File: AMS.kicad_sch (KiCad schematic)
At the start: 1 part

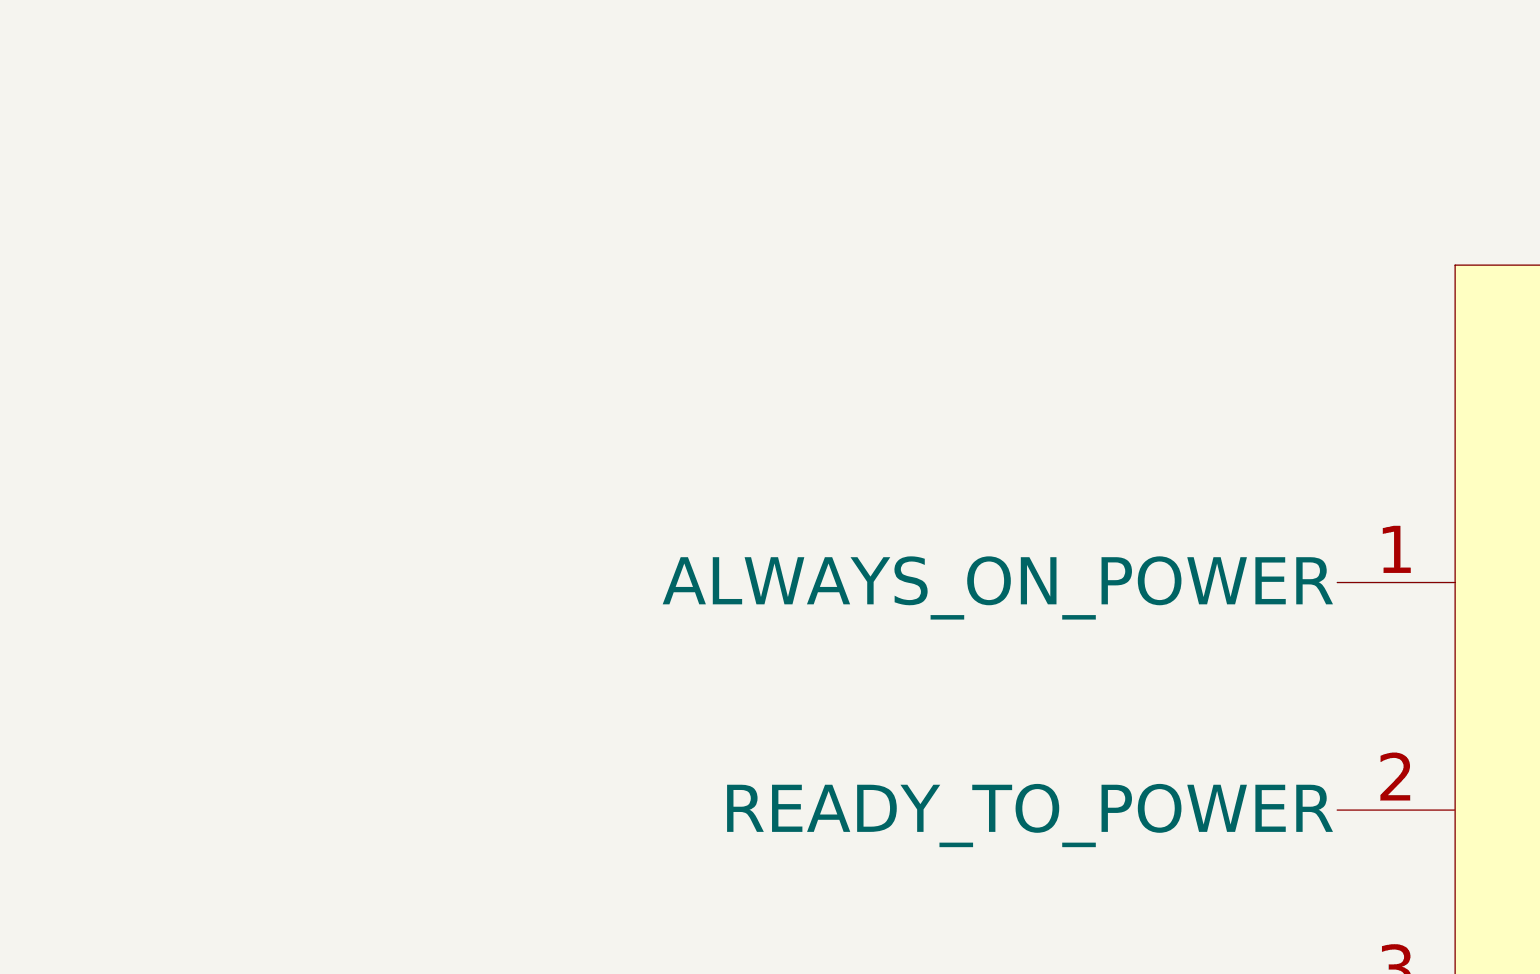
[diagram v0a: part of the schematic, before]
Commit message: update
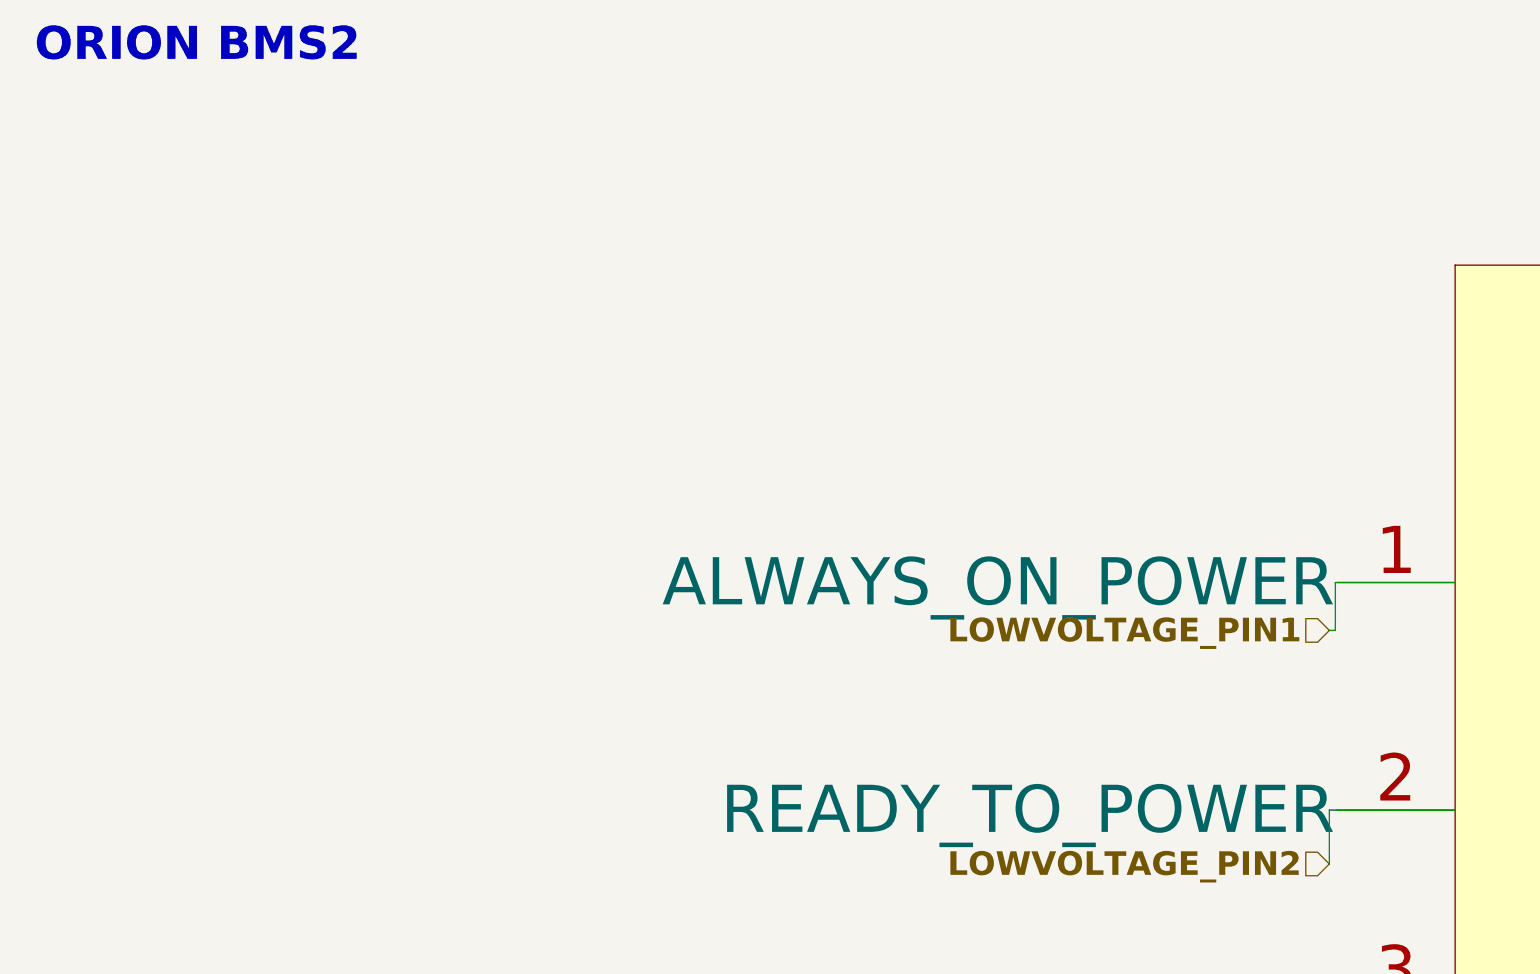
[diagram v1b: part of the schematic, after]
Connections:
- net LOWVOLTAGE_PIN1: now reaches BMS1.1 (ALWAYS_ON_POWER)
- net LOWVOLTAGE_PIN2: now reaches BMS1.2 (READY_TO_POWER)
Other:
- note added: "ORION BMS2"
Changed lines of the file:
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@@
 	(generator_version "8.0")
 	(paper "A0")
+	(wire
+		(pts
+			(xy 477.52 215.9) (xy 477.52 204.47)
+		)
+		(stroke
+			(width 0)
+			(type default)
+		)
+	)
+	(wire
+		(pts
+			(xy 477.52 166.37) (xy 478.79 166.37)
+		)
+		(stroke
+			(width 0)
+			(type default)
+		)
+	)
+	(wire
+		(pts
+			(xy 478.79 166.37) (xy 478.79 156.21)
+		)
+		(stroke
+			(width 0)
+			(type default)
+		)
+	)
+	(wire
+		(pts
+			(xy 478.79 156.21) (xy 504.19 156.21)
+		)
+		(stroke
+			(width 0)
+			(type default)
+		)
+	)
+	(wire
+		(pts
+			(xy 477.52 204.47) (xy 504.19 204.47)
+		)
+		(stroke
+			(width 0)
+			(type default)
+		)
+	)
 	(image
 		(at 180.34 106.68)
@@
 		)
 	)
+	(text "ORION BMS2"
+		(exclude_from_sim no)
+		(at 237.49 42.164 0)
+		(effects
+			(font
+				(size 7 7)
+				(thickness 1.4)
+				(bold yes)
+			)
+		)
+	)
+	(hierarchical_label "LOWVOLTAGE_PIN1"
+		(shape input)
+		(at 477.52 166.37 180)
+		(fields_autoplaced yes)
+		(effects
+			(font
+				(size 5 5)
+				(bold yes)
+			)
+			(justify right)
+		)
+	)
+	(hierarchical_label "LOWVOLTAGE_PIN2"
+		(shape input)
+		(at 477.52 215.9 180)
+		(fields_autoplaced yes)
+		(effects
+			(font
+				(size 5 5)
+				(bold yes)
+			)
+			(justify right)
+		)
+	)
